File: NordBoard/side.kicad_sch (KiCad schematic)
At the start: 39 parts, among them SW15 SW_Push, SW16 SW_Push, SW2 SW_Push, SW22 SW_Push, SW23 SW_Push, SW24 SW_Push, SW25 SW_Push, SW26 SW_Push, SW27 SW_Push, SW28 SW_Push, SW29 SW_Push, SW30 SW_Push, SW31 SW_Push, SW32 SW_Push, SW33 SW_Push, SW34 SW_Push, SW9 SW_Push, U1 MOUDLE-SEEEDUINO-XIAO

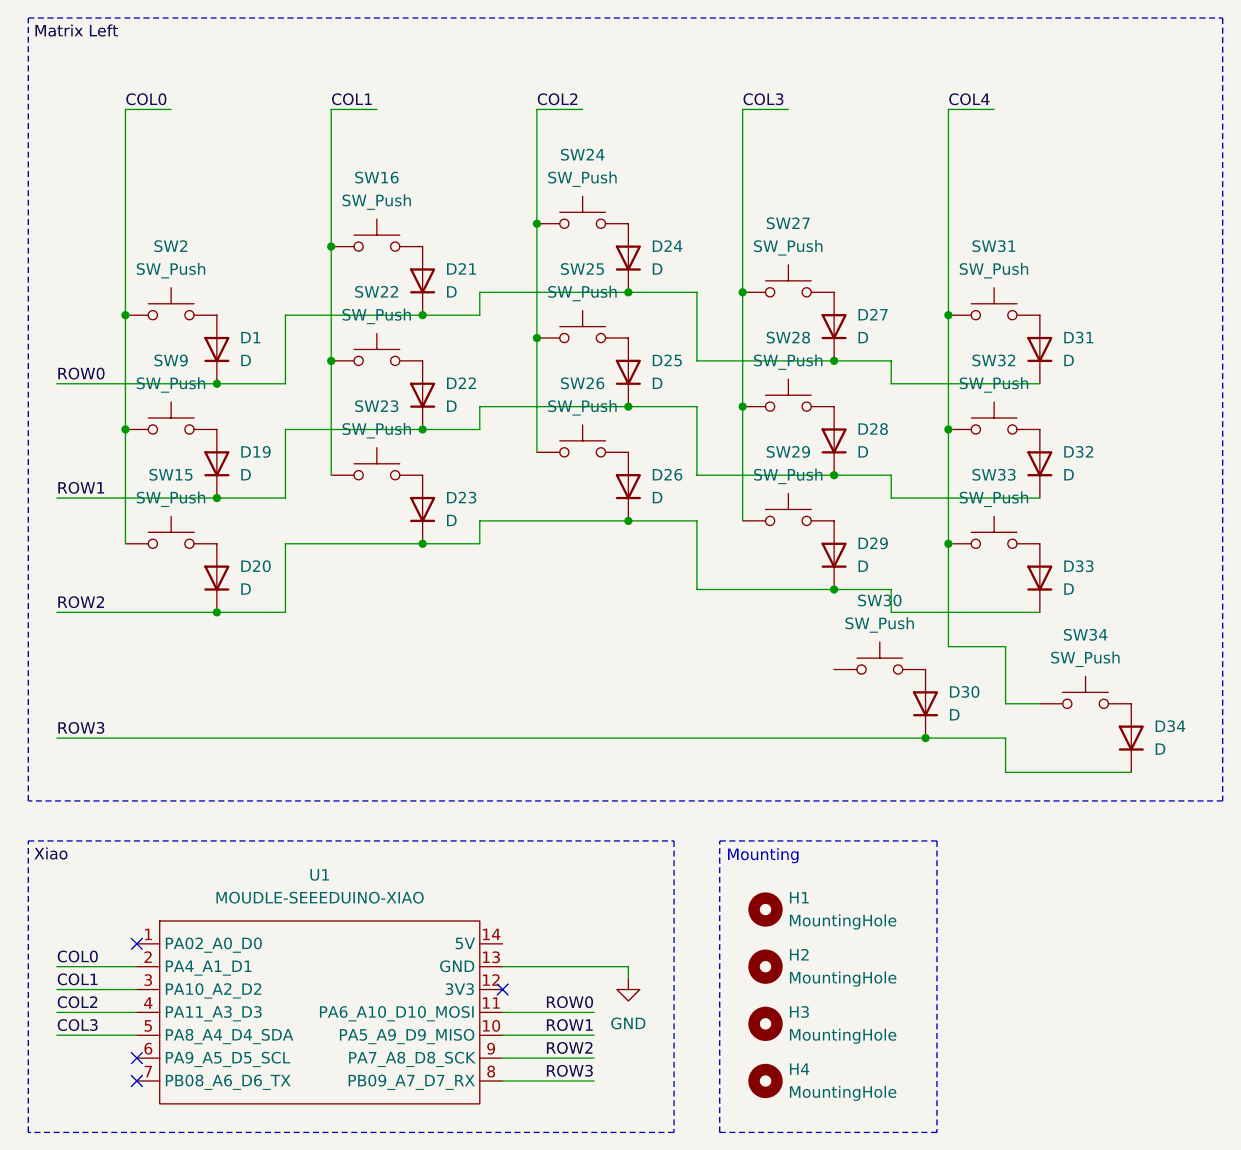
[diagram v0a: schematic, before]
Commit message: feat: finish schem, finish PCB layout
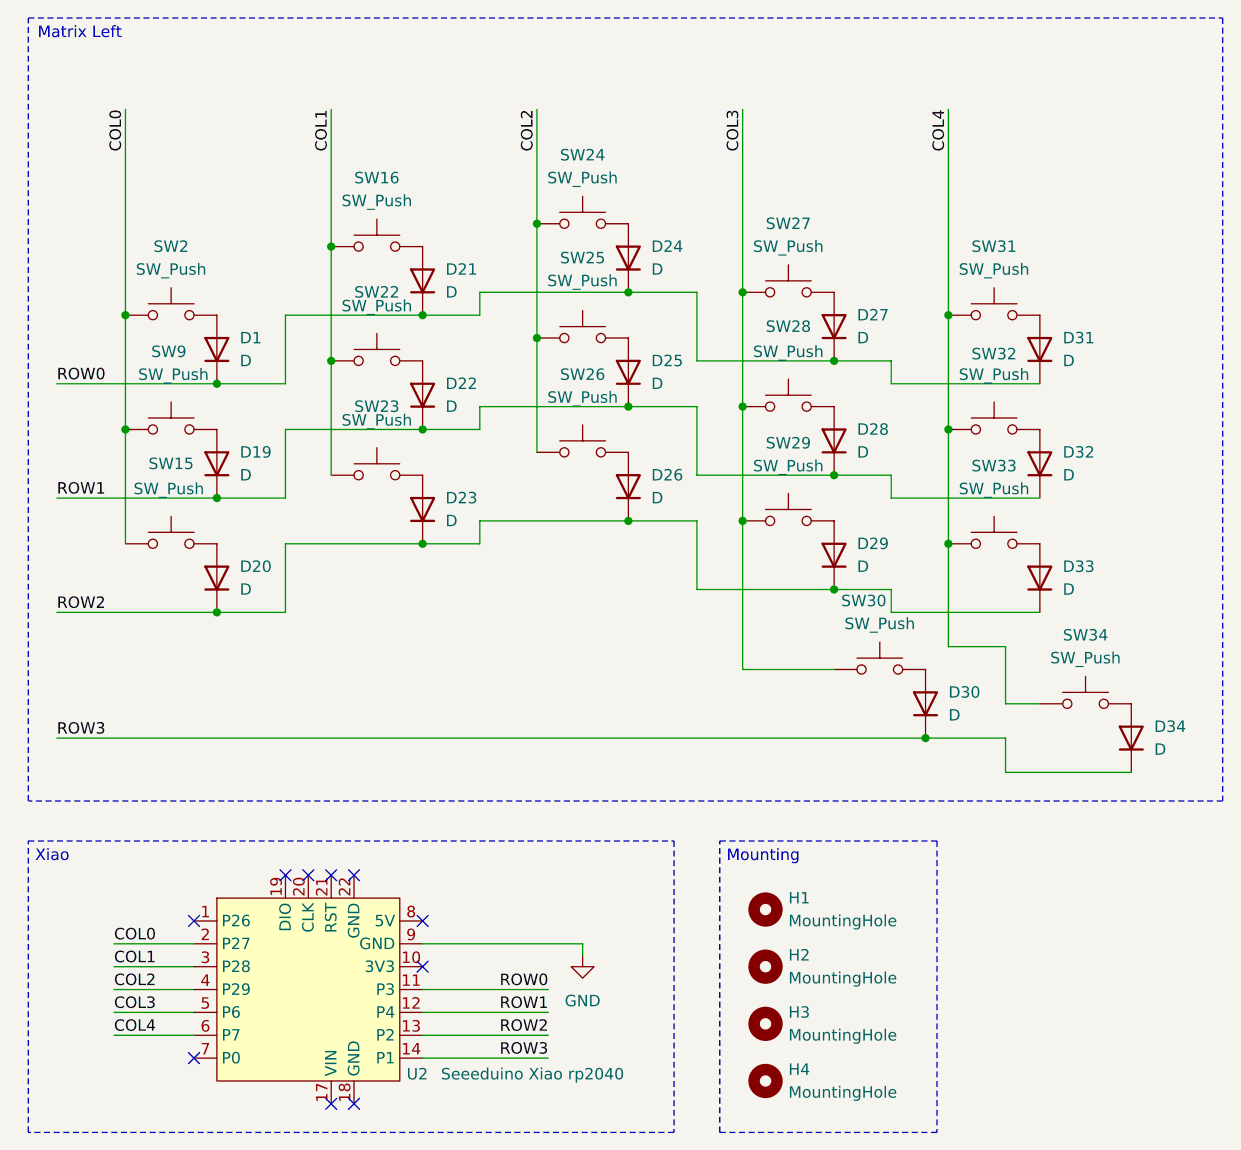
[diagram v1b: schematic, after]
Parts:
- removed U1: MOUDLE-SEEEDUINO-XIAO, Seeed Studio XIAO Series Library:XIAO-RP2040-DIP, symbol XIAO_RP2040:MOUDLE-SEEEDUINO-XIAO
- added U2: Seeeduino Xiao rp2040, PCM_marbastlib-xp-promicroish:Xiao_rp2040_ACH, symbol PCM_marbastlib-promicroish:Seeeduino_Xiao_rp2040
- D1, D19, D20, D21, D22, D23, D24, D25, D26, D27, D28, D29, D30, D31, D32, D33, D34: footprint (none) -> Diode_SMD:D_SMA-SMB_Universal_Handsoldering
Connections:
- net COL0: now also U2.2 (P27)
- net COL1: now also U2.3 (P28)
- net COL2: now also U2.4 (P29)
- net COL3: now also SW30.1, U2.5 (P6)
- net COL4: now also U2.6 (P7)
- net GND: now also U2.9 (GND)
- net ROW0: now also U2.11 (P3)
- net ROW1: now also U2.12 (P4)
- net ROW2: now also U2.13 (P2)
- net ROW3: now also U2.14 (P1)
- no-connect marks 4 -> 10
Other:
- note added: "Matrix Left"
- note added: "Xiao"
